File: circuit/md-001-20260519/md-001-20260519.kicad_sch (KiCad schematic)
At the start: 11 parts, among them J1 VIN-motor

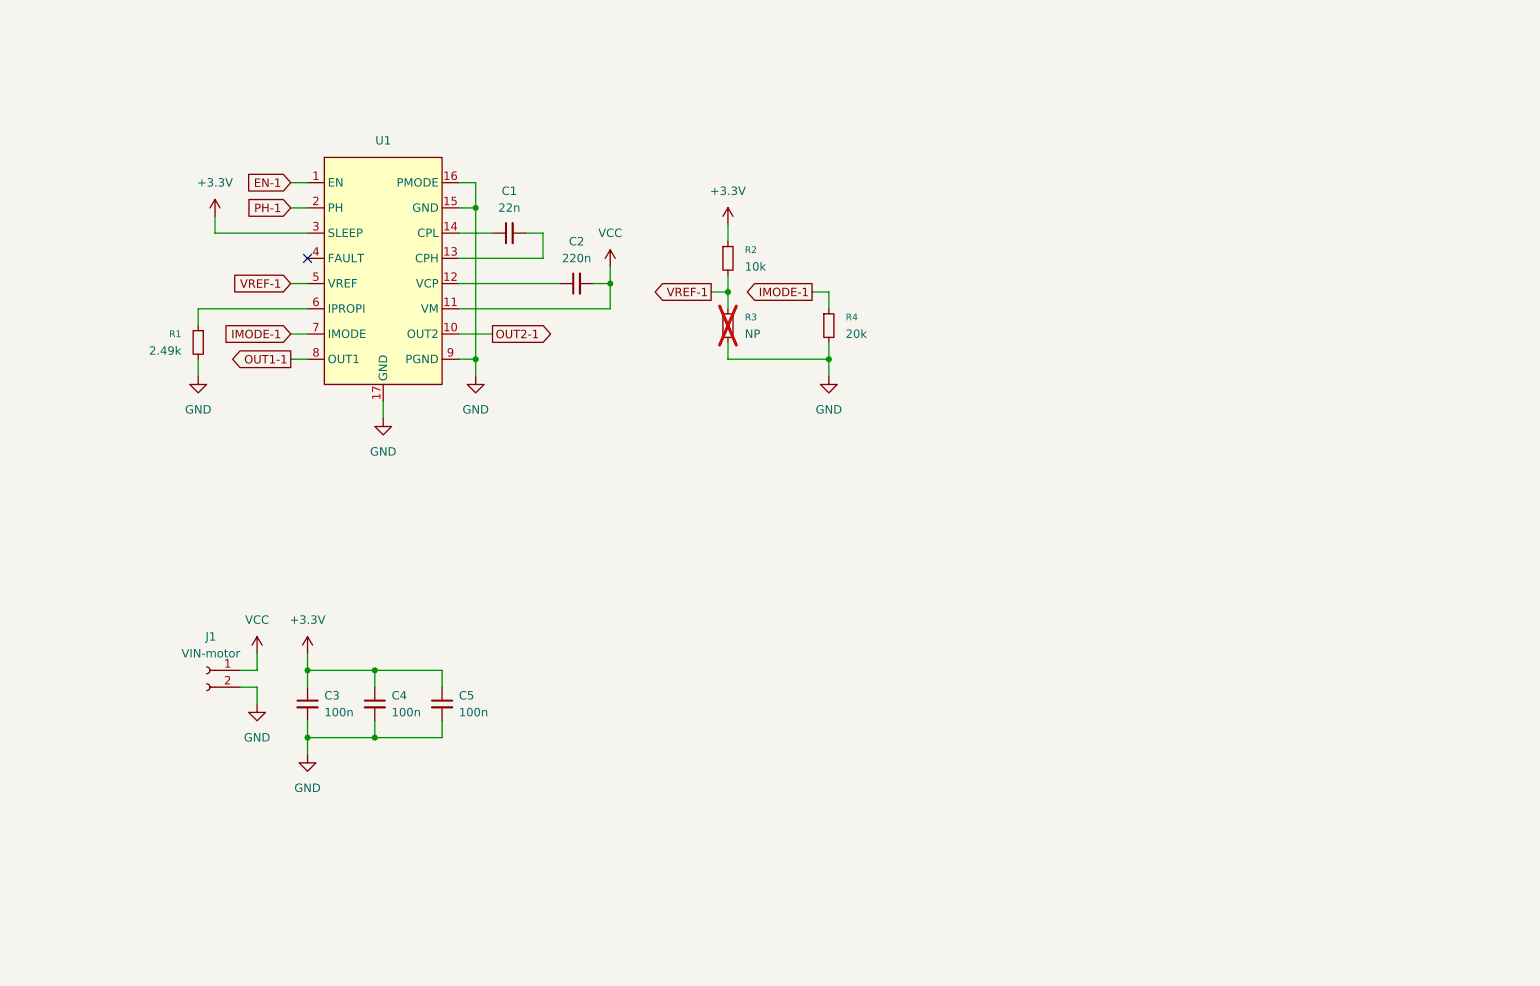
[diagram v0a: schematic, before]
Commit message: Update MD基板を更新
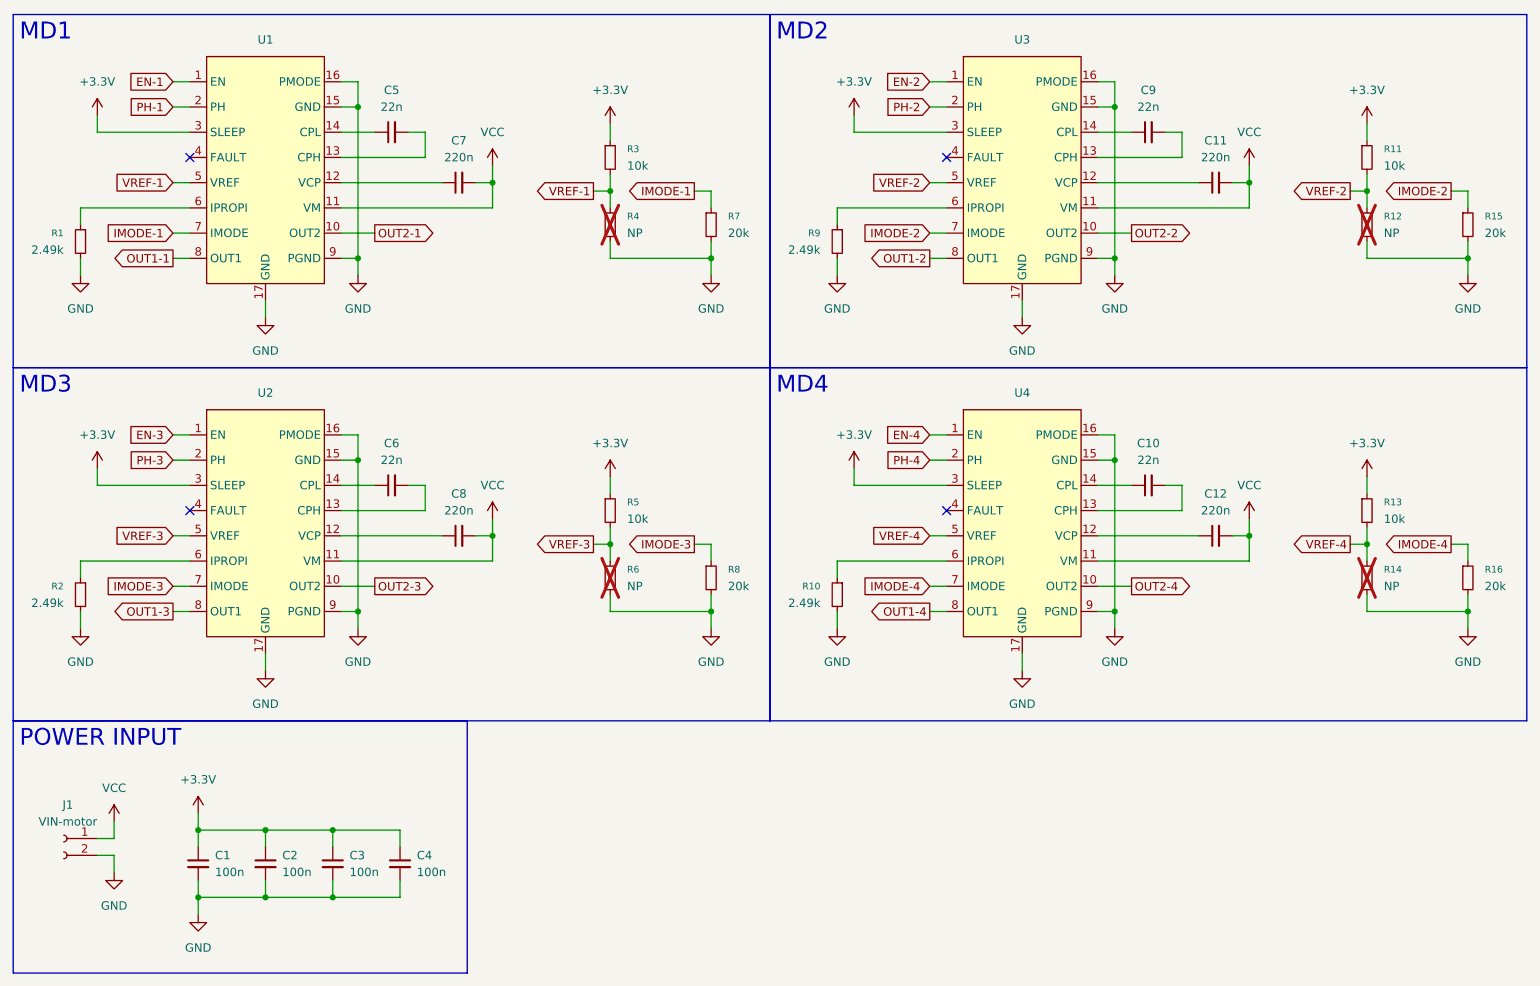
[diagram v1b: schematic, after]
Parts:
- added C10, C6, C9: 22n, symbol Device:C_Small
- added C11, C12, C8: 220n, symbol Device:C_Small
- added C4: 100n, symbol Device:C_Small
- added R10, R2, R9: 2.49k, symbol Device:R_Small
- added R11, R13, R5: 10k, symbol Device:R_Small
- added R12, R14, R6: NP, symbol Device:R_Small
- added R15, R16, R8: 20k, symbol Device:R_Small
- added U2, U3, U4: (no value), symbol @Thrive_symbol_md:DRV8874
- renumbered C3 to C1, C4 to C2, C5 to C3, C1 to C5, C2 to C7, R2 to R3, R3 to R4, R4 to R7
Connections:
- net +3.3V: now also C4.1, R11.1, R13.1, R5.1, U2.3 (SLEEP), U3.3 (SLEEP), U4.3 (SLEEP)
- net GND: now also C4.2, R10.2, R12.2, R14.2, R15.2, R16.2, R2.2, R6.2, R8.2, R9.2, U2.15 (GND), U2.16 (PMODE), U2.17 (GND), U2.9 (PGND), U3.15 (GND), U3.16 (PMODE), U3.17 (GND), U3.9 (PGND), U4.15 (GND), U4.16 (PMODE), U4.17 (GND), U4.9 (PGND)
- net VCC: now also C11.2, C12.2, C8.2, U2.11 (VM), U3.11 (VM), U4.11 (VM)
- new net: C12.1, U4.12 (VCP)
- new net: C10.2, U4.13 (CPH)
- new net: C10.1, U4.14 (CPL)
- new net: R10.1, U4.6 (IPROPI)
- new net: C11.1, U3.12 (VCP)
- new net: C9.2, U3.13 (CPH)
- new net: C9.1, U3.14 (CPL)
- new net: R9.1, U3.6 (IPROPI)
- new net: C8.1, U2.12 (VCP)
- new net: C6.2, U2.13 (CPH)
- new net: C6.1, U2.14 (CPL)
- new net: R2.1, U2.6 (IPROPI)
- new net EN-2: U3.1 (EN)
- new net EN-3: U2.1 (EN)
- new net EN-4: U4.1 (EN)
- new net IMODE-2: R15.1, U3.7 (IMODE)
- new net IMODE-3: R8.1, U2.7 (IMODE)
- new net IMODE-4: R16.1, U4.7 (IMODE)
- new net OUT1-2: U3.8 (OUT1)
- new net OUT1-3: U2.8 (OUT1)
- new net OUT1-4: U4.8 (OUT1)
- new net OUT2-2: U3.10 (OUT2)
- new net OUT2-3: U2.10 (OUT2)
- new net OUT2-4: U4.10 (OUT2)
- new net PH-2: U3.2 (PH)
- new net PH-3: U2.2 (PH)
- new net PH-4: U4.2 (PH)
- new net VREF-2: R11.2, R12.1, U3.5 (VREF)
- new net VREF-3: R5.2, R6.1, U2.5 (VREF)
- new net VREF-4: R13.2, R14.1, U4.5 (VREF)
- no-connect marks 1 -> 4
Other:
- moved on the sheet: C1, C2, C3, C5, C7, J1, R1, R3, R4, R7, U1
